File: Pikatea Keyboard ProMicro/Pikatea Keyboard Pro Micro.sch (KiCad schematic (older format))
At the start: 153 parts, among them SW2 Rotary_Encoder_Switch, U2 Teensy2.0_(Arduino)

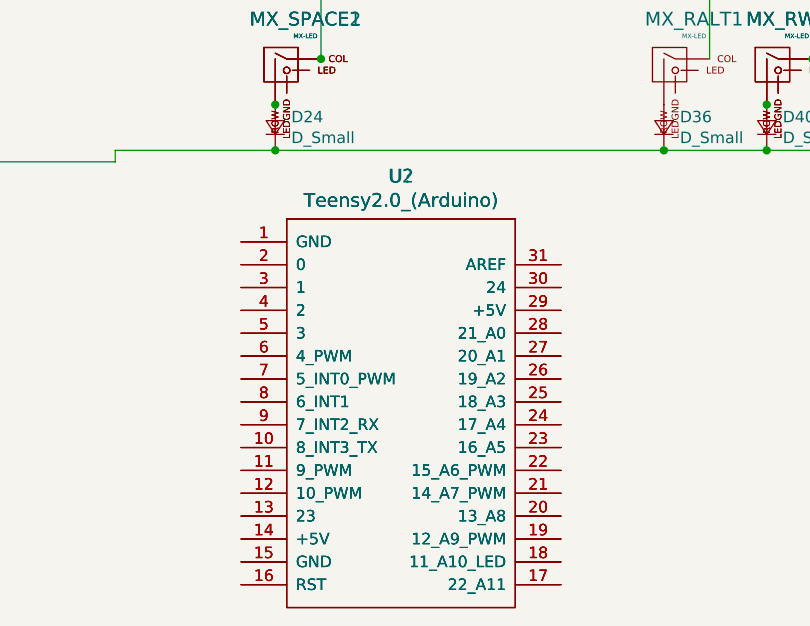
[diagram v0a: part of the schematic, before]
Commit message: updates
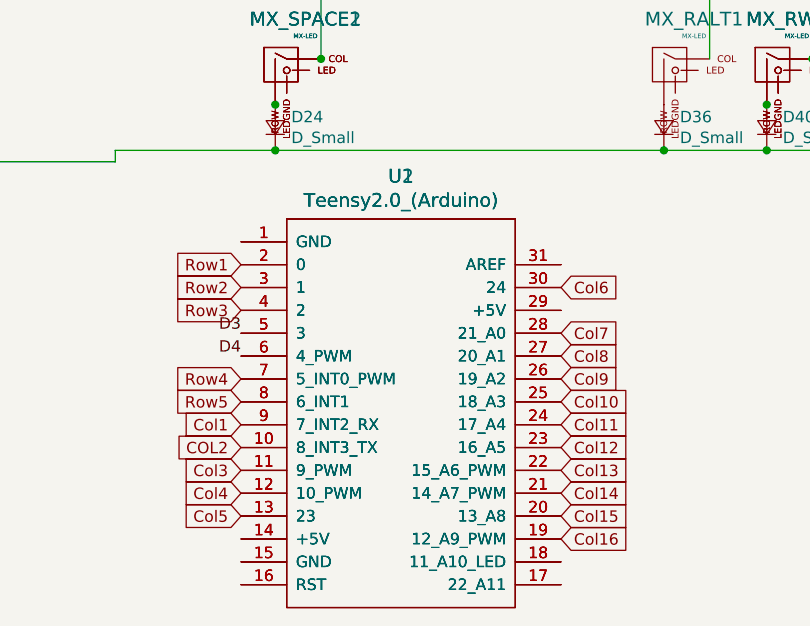
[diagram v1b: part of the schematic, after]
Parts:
- gave numbers to parts that had none: 1
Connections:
- net COL2: now also U1.10 (8_INT3_TX), U2.10 (8_INT3_TX)
- net Col1: now also U1.9 (7_INT2_RX), U2.9 (7_INT2_RX)
- net Col10: now also U1.25 (18_A3), U2.25 (18_A3)
- net Col11: now also U1.24 (17_A4), U2.24 (17_A4)
- net Col12: now also U1.23 (16_A5), U2.23 (16_A5)
- net Col13: now also U1.22 (15_A6_PWM), U2.22 (15_A6_PWM)
- net Col14: now also U1.21 (14_A7_PWM), U2.21 (14_A7_PWM)
- net Col15: now also U1.20 (13_A8), U2.20 (13_A8)
- net Col16: now also U1.19 (12_A9_PWM), U2.19 (12_A9_PWM)
- net Col3: now also U1.11 (9_PWM), U2.11 (9_PWM)
- net Col4: now also U1.12 (10_PWM), U2.12 (10_PWM)
- net Col5: now also U1.13 (23), U2.13 (23)
- net Col6: now also U1.30 (24), U2.30 (24)
- net Col7: now also U1.28 (21_A0), U2.28 (21_A0)
- net Col8: now also U1.27 (20_A1), U2.27 (20_A1)
- net Col9: now also U1.26 (19_A2), U2.26 (19_A2)
- net D3: now also U1.5 (3), U2.5 (3)
- net D4: now also U1.6 (4_PWM), U2.6 (4_PWM)
- net Row1: now also U1.2 (0), U2.2 (0)
- net Row2: now also U1.3 (1), U2.3 (1)
- net Row3: now also U1.4 (2), U2.4 (2)
- net Row4: now also U1.7 (5_INT0_PWM), U2.7 (5_INT0_PWM)
- net Row5: now also U1.8 (6_INT1), U2.8 (6_INT1)
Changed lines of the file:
@@
 $EndComp
 $Comp
-L teensy:Teensy2.0_(Arduino) U?
+L teensy:Teensy2.0_(Arduino) U1
 U 1 1 60F49BE0
 P 4750 6600
-F 0 "U?" H 4750 7637 60  0000 C CNN
+F 0 "U1" H 4750 7637 60  0000 C CNN
 F 1 "Teensy2.0_(Arduino)" H 4750 7531 60  0000 C CNN
 F 2 "teensy:Teensy2.0" H 4850 5550 60  0001 C CNN
@@
 	1    0    0    -1
 $EndComp
+Text GLabel 4050 5950 0    50   Input ~ 0
+Row1
+Text Label 4050 6250 2    50   ~ 0
+D3
+Text Label 4050 6350 2    50   ~ 0
+D4
+Text GLabel 4050 6050 0    50   Input ~ 0
+Row2
+Text GLabel 4050 6150 0    50   Input ~ 0
+Row3
+Text GLabel 4050 6450 0    50   Input ~ 0
+Row4
+Text GLabel 4050 6550 0    50   Input ~ 0
+Row5
+Text GLabel 4050 6650 0    50   Input ~ 0
+Col1
+Text GLabel 4050 6750 0    50   Input ~ 0
+COL2
+Text GLabel 4050 6850 0    50   Input ~ 0
+Col3
+Text GLabel 4050 6950 0    50   Input ~ 0
+Col4
+Text GLabel 4050 7050 0    50   Input ~ 0
+Col5
+Text GLabel 5450 6050 2    50   Input ~ 0
+Col6
+Text GLabel 5450 6250 2    50   Input ~ 0
+Col7
+Text GLabel 5450 6350 2    50   Input ~ 0
+Col8
+Text GLabel 5450 6450 2    50   Input ~ 0
+Col9
+Text GLabel 5450 6550 2    50   Input ~ 0
+Col10
+Text GLabel 5450 6650 2    50   Input ~ 0
+Col11
+Text GLabel 5450 6750 2    50   Input ~ 0
+Col12
+Text GLabel 5450 6850 2    50   Input ~ 0
+Col13
+Text GLabel 5450 6950 2    50   Input ~ 0
+Col14
+Text GLabel 5450 7050 2    50   Input ~ 0
+Col15
+Text GLabel 5450 7150 2    50   Input ~ 0
+Col16
 $EndSCHEMATC
